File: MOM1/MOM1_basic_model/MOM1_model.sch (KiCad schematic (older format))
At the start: 4 parts, among them J2 5-5530843-4, J3 5-5530843-4, J4 5-5530843-4, J5 5-5530843-4

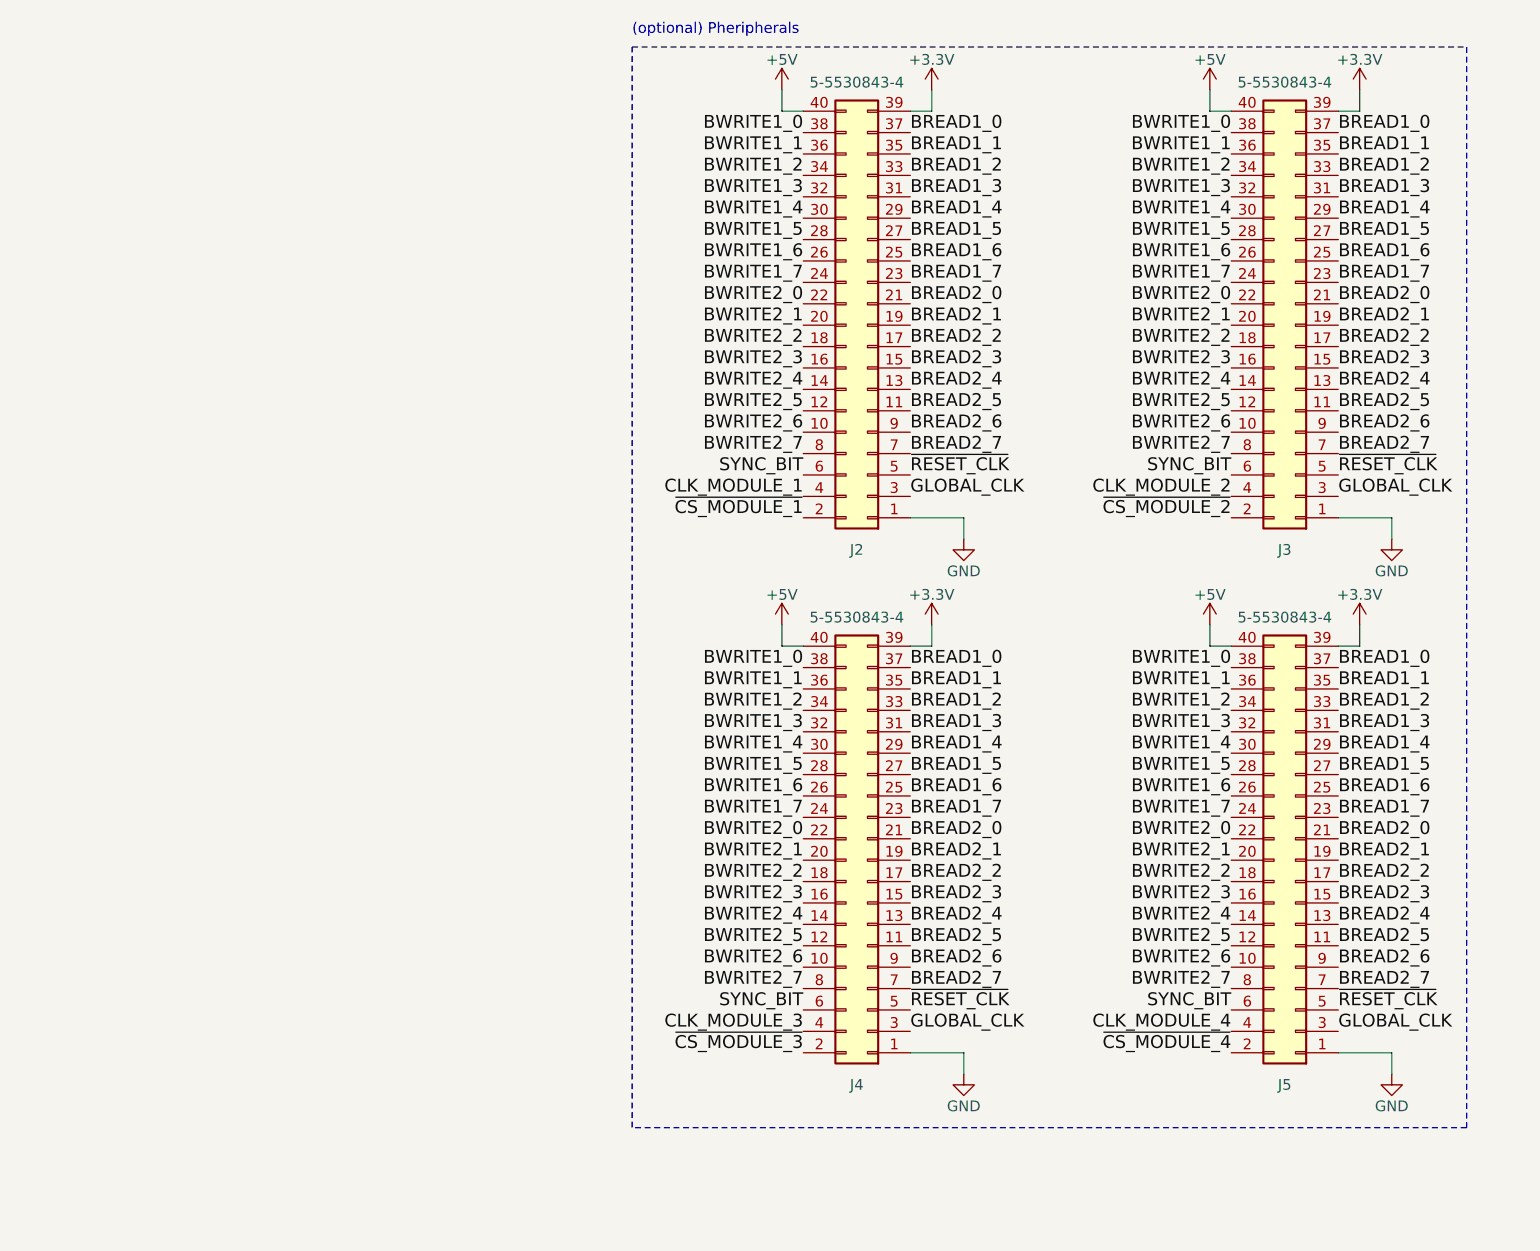
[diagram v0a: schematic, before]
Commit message: Made plenty of change (see CHANGELOG file)
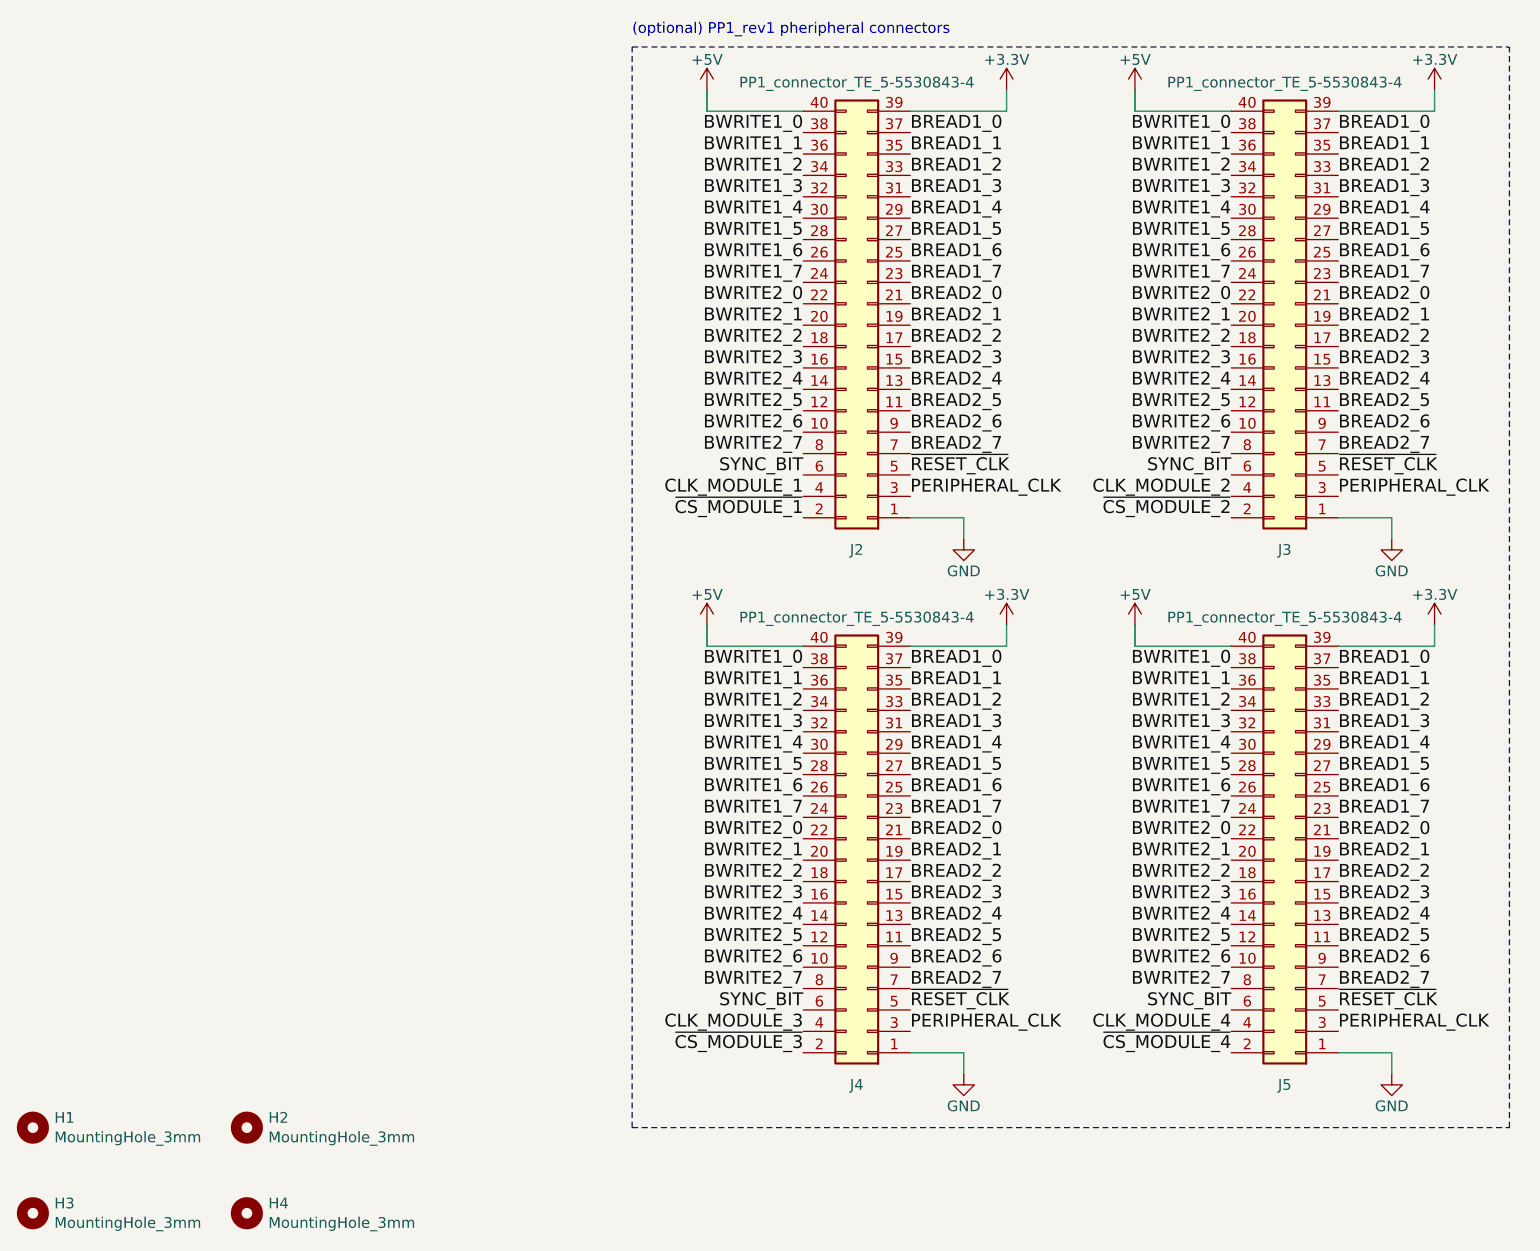
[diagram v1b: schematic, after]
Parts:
- added H1, H2, H3, H4: MountingHole_3mm, MountingHole:MountingHole_3mm, symbol Mechanical:MountingHole
- J2, J3, J4, J5: value 5-5530843-4 -> PP1_connector_TE_5-5530843-4; footprint Eurocard:SHDR40W89P485X254_2X20_5740X935X1562P -> TE_5-5530843-4:TE_5-5530843-4
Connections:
- net GLOBAL_CLK renamed PERIPHERAL_CLK
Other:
- note added: "(optional) PP1_rev1 pheripheral connectors"
- note removed: "(optional) Pheripherals"
